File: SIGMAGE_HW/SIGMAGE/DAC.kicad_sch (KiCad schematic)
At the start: 40 parts, among them J20 SJ63073E, J21 SJ63073E, U10 PCM5102APWR, U3 PCM5102APWR

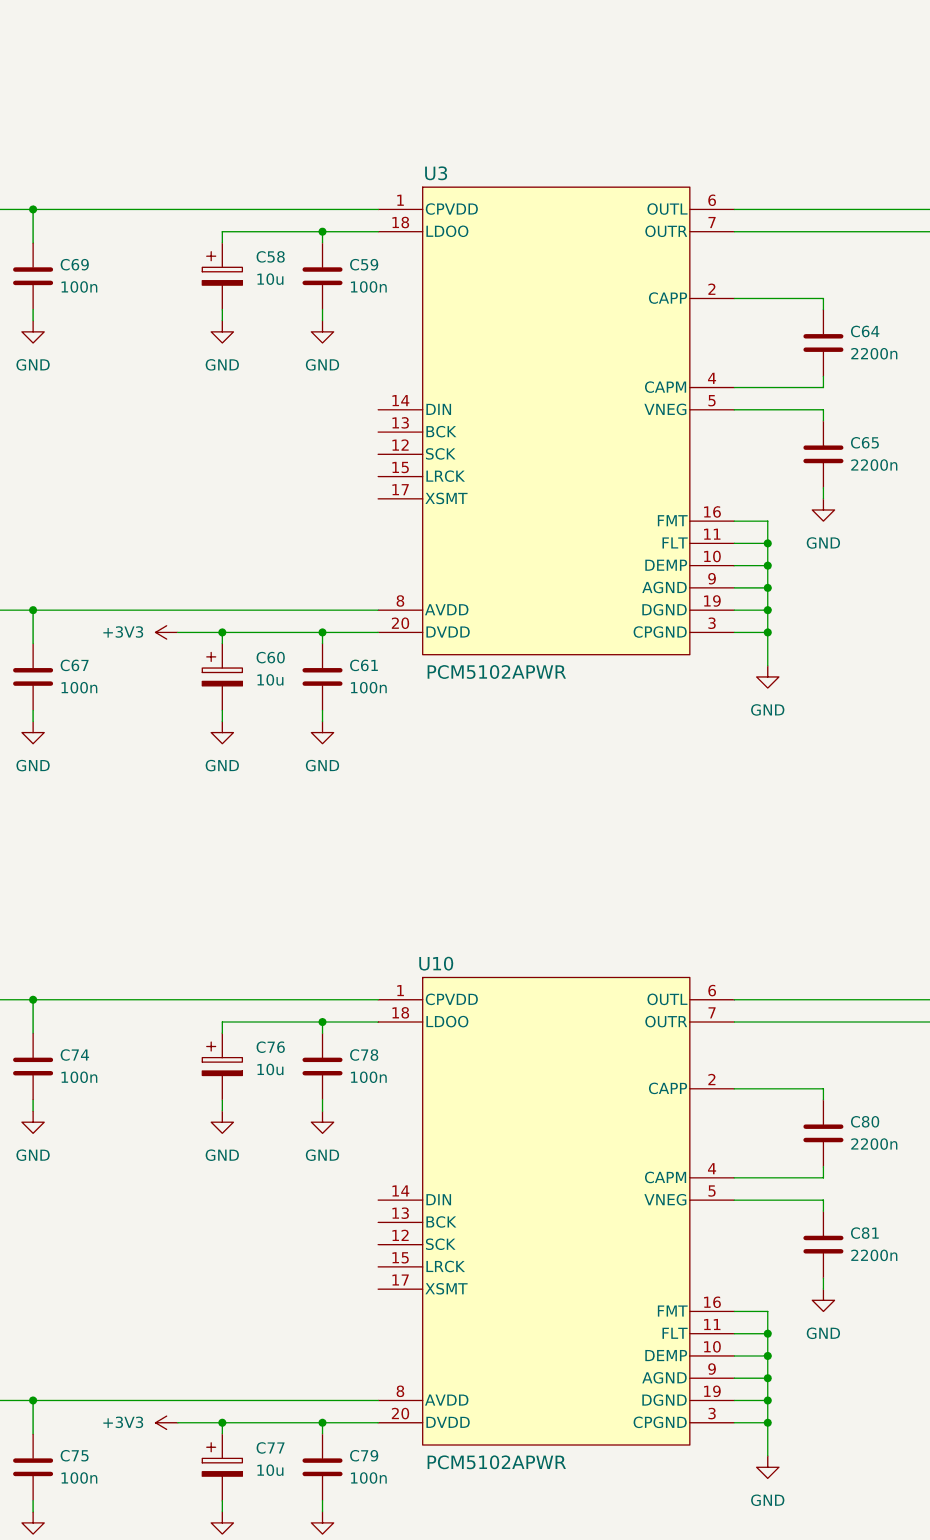
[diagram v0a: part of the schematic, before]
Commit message: preps for FPGA
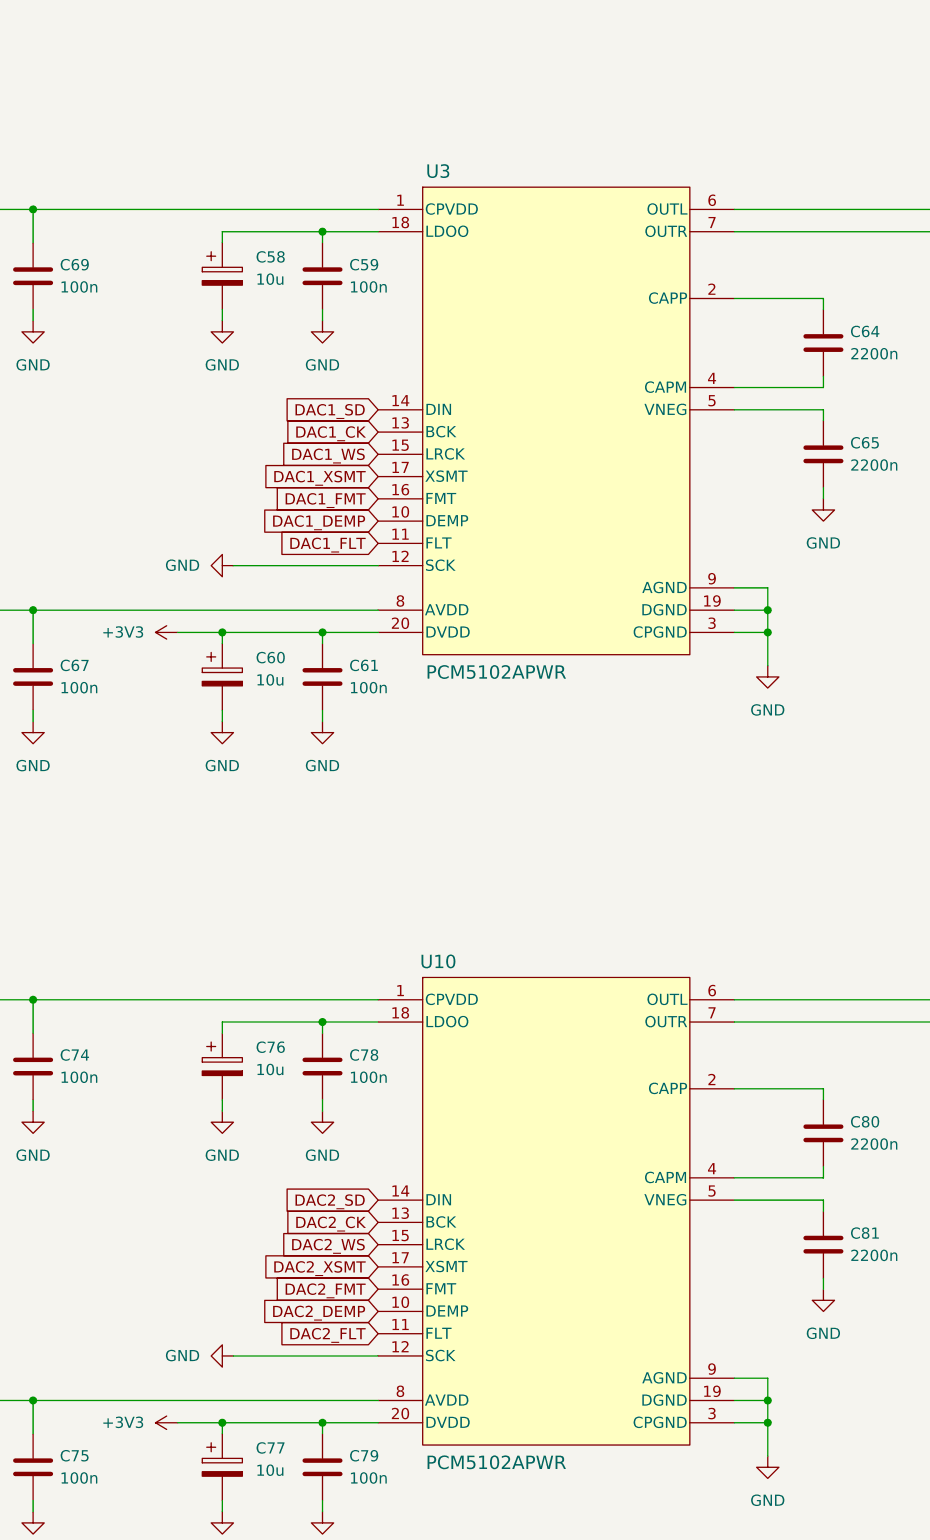
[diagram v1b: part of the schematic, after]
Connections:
- net GND: now also U10.12 (SCK), U3.12 (SCK); no longer U10.10 (DEMP), U10.11 (FLT), U10.16 (FMT), U3.10 (DEMP), U3.11 (FLT), U3.16 (FMT)
- net DAC1_CK: now reaches U3.13 (BCK)
- net DAC1_SD: now reaches U3.14 (DIN)
- net DAC1_WS: now reaches U3.15 (LRCK)
- net DAC1_XSMT: now reaches U3.17 (XSMT)
- net DAC2_CK: now reaches U10.13 (BCK)
- net DAC2_SD: now reaches U10.14 (DIN)
- net DAC2_WS: now reaches U10.15 (LRCK)
- net DAC2_XSMT: now reaches U10.17 (XSMT)
- new net DAC1_DEMP: U3.10 (DEMP)
- new net DAC1_FLT: U3.11 (FLT)
- new net DAC1_FMT: U3.16 (FMT)
- new net DAC2_DEMP: U10.10 (DEMP)
- new net DAC2_FLT: U10.11 (FLT)
- new net DAC2_FMT: U10.16 (FMT)

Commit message: major changes
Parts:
- added C145, C146, C147, C148, C153, C154, C155, C156: 10u, Capacitor_SMD:C_0603_1608Metric, symbol Device:C_Polarized
- added C149, C150, C151, C152, C157, C158, C159, C160: 100n, Capacitor_SMD:C_0603_1608Metric, symbol Device:C
- added C161, C162, C163, C164: 2200n, Capacitor_SMD:C_0603_1608Metric, symbol Device:C
- added C165, C166, C167, C168: 1u, Capacitor_SMD:C_1206_3216Metric, symbol Device:C
- added C169, C170, C171, C172: 10n, Capacitor_SMD:C_0603_1608Metric, symbol Device:C
- added J24, J25: SJ63073E, SIGMAGE:SJ63073E, symbol SIGMAGE:SJ63073E
- added R52, R53, R54, R55: 1M, Resistor_SMD:R_0603_1608Metric, symbol Device:R
- added R63, R64, R65, R66: 100, Resistor_SMD:R_0603_1608Metric, symbol Device:R
- added U20, U21: PCM5102APWR, SIGMAGE:PCM5102APWR, symbol SIGMAGE:PCM5102APWR
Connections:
- net GND: now also C145.2, C146.2, C147.2, C148.2, C149.2, C150.2, C151.2, C152.2, C153.2, C154.2, C155.2, C156.2, C157.2, C158.2, C159.2, C160.2, C162.2, C164.2, C169.2, C170.2, C171.2, C172.2, J24.1 (SLEEVE), J25.1 (SLEEVE), R52.1, R53.1, R54.1, R55.1, U20.12 (SCK), U20.19 (DGND), U20.3 (CPGND), U20.9 (AGND), U21.12 (SCK), U21.19 (DGND), U21.3 (CPGND), U21.9 (AGND)
- net Use film cap here!: now also C82.2, C84.1, J21.2 (TIP), R37.2, R39.1, R39.2
- net +3V3 renamed AVCC_3V3
- net AVCC_3V3: now also C145.1, C146.1, C147.1, C148.1, C149.1, C150.1, C151.1, C152.1, U20.1 (CPVDD), U20.8 (AVDD), U21.1 (CPVDD), U21.8 (AVDD); no longer C60.1, C61.1, C77.1, C79.1, U10.20 (DVDD), U3.20 (DVDD)
- new net: C153.1, C157.1, U20.18 (LDOO)
- new net: C161.1, U20.2 (CAPP)
- new net: C161.2, U20.4 (CAPM)
- new net: C162.1, U20.5 (VNEG)
- new net: C165.1, U20.6 (OUTL)
- new net: C166.1, U20.7 (OUTR)
- new net: C169.1, J24.2 (TIP), R63.2
- new net: C170.1, J24.3 (RING), R64.2
- new net: C166.2, R53.2, R64.1
- new net: C165.2, R52.2, R63.1
- new net: C155.1, C159.1, U21.18 (LDOO)
- new net: C167.2, R54.2, R65.1
- new net: C168.1, U21.7 (OUTR)
- new net: C168.2, R55.2, R66.1
- new net: C163.1, U21.2 (CAPP)
- new net: C163.2, U21.4 (CAPM)
- new net: C172.1, J25.3 (RING), R66.2
- new net: C171.1, J25.2 (TIP), R65.2
- new net: C164.1, U21.5 (VNEG)
- new net: C167.1, U21.6 (OUTL)
- new net DAC3_CK: U20.13 (BCK)
- new net DAC3_DEMP: U20.10 (DEMP)
- new net DAC3_FLT: U20.11 (FLT)
- new net DAC3_FMT: U20.16 (FMT)
- new net DAC3_SD: U20.14 (DIN)
- new net DAC3_WS: U20.15 (LRCK)
- new net DAC3_XSMT: U20.17 (XSMT)
- new net DAC4_CK: U21.13 (BCK)
- new net DAC4_DEMP: U21.10 (DEMP)
- new net DAC4_FLT: U21.11 (FLT)
- new net DAC4_FMT: U21.16 (FMT)
- new net DAC4_SD: U21.14 (DIN)
- new net DAC4_WS: U21.15 (LRCK)
- new net DAC4_XSMT: U21.17 (XSMT)
- new net DVCC_3V3: C154.1, C156.1, C158.1, C160.1, C60.1, C61.1, C77.1, C79.1, U10.20 (DVDD), U20.20 (DVDD), U21.20 (DVDD), U3.20 (DVDD)
- no-connect marks 6 -> 12
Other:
- moved on the sheet: C58, C59, C60, C61, C62, C63, C64, C65, C66, C67, C68, C69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
